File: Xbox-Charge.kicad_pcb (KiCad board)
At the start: 4 copper layers, 38.5 x 38.5 mm, 66 parts, among them J1 Conn_01x04_Pin, Q1 CSD17551Q3A, Q2 CSD17551Q3A, Q3 CSD17551Q3A, Q4 CSD17551Q3A, Q5 CSD25402Q3A, U2 BQ25713RSNR

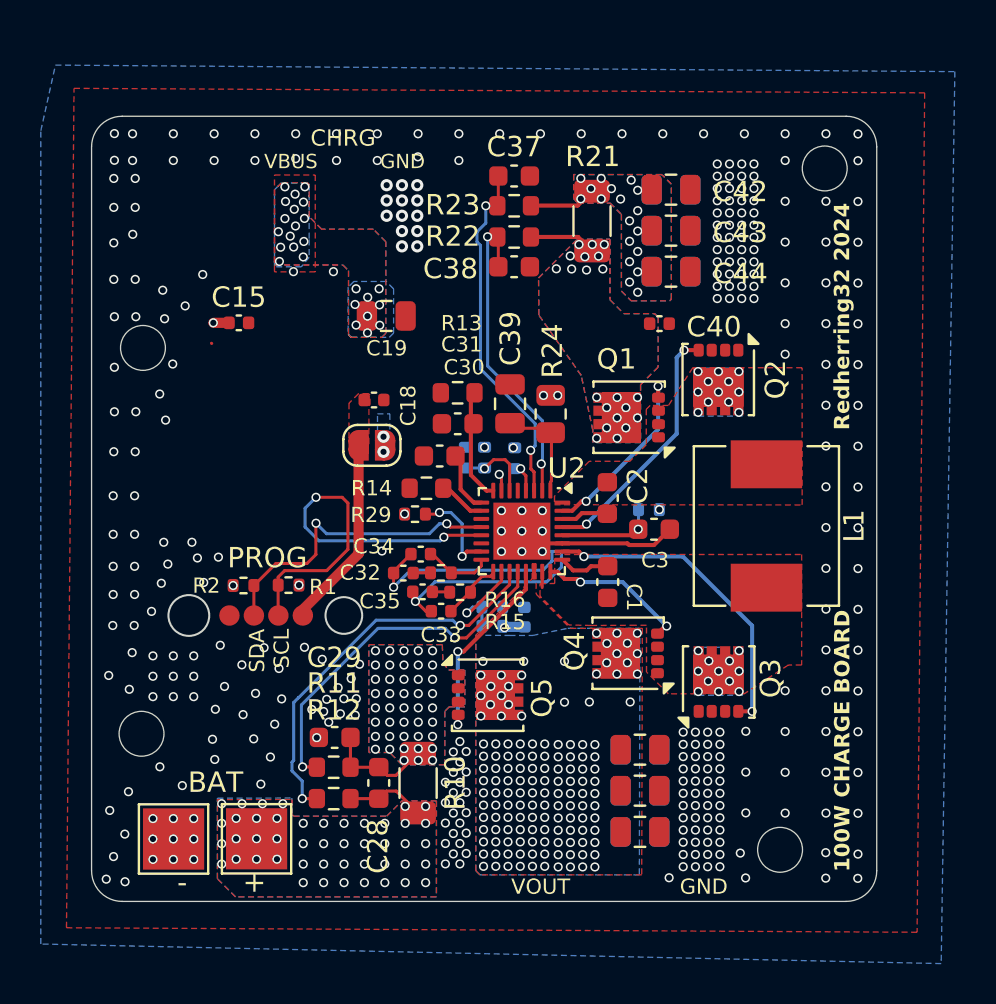
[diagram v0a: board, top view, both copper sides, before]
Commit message: Trim corner
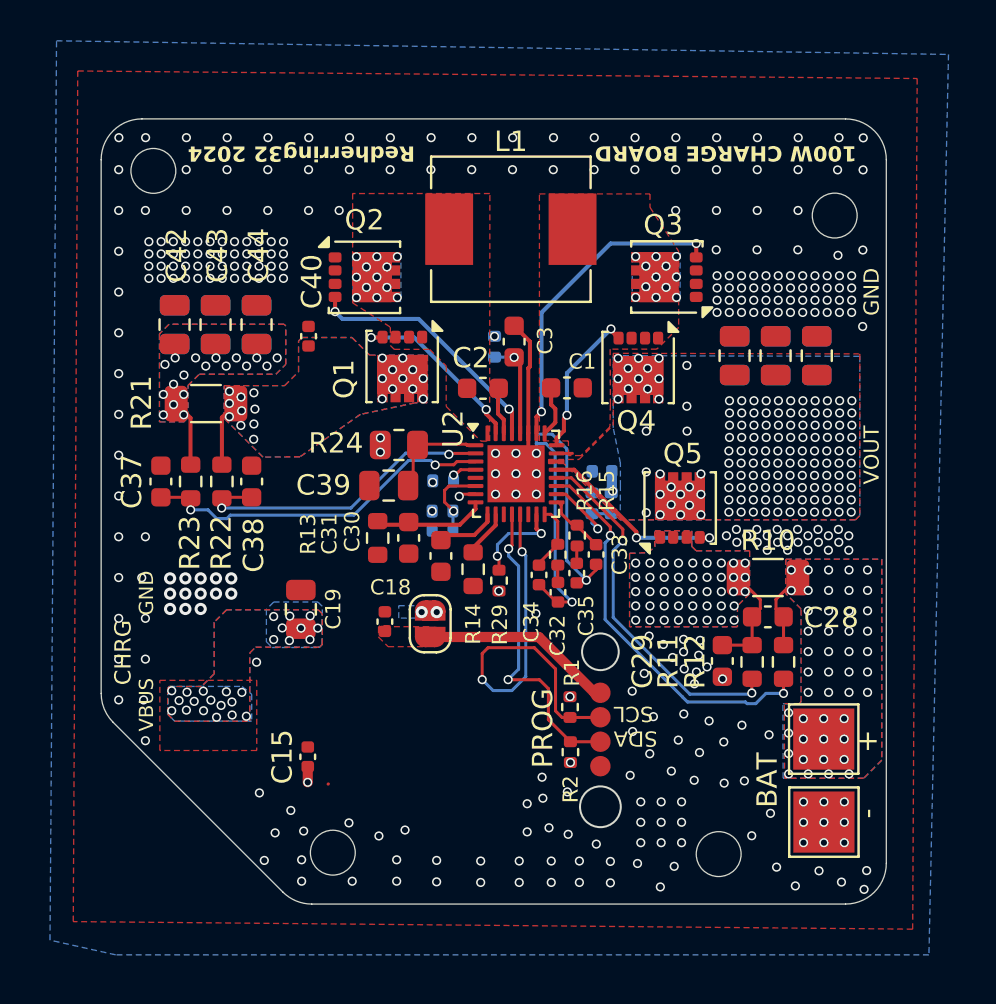
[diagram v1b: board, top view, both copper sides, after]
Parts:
- moved REF** 32.9 mm to (150.8, 33.3), turned to 90 degrees
- moved TP3 31.9 mm to (183.7, 65.2), turned to 90 degrees
- moved REF** 31.2 mm to (184.2, 35.5), turned to 90 degrees
- moved REF** 28.9 mm to (178.5, 66.8), turned to 90 degrees
- moved TP2 28.2 mm to (183.7, 61.2), turned to 90 degrees
- moved REF** 26.4 mm to (159.6, 66.7), turned to 90 degrees
- moved C42 25.2 mm to (151.8, 40.8), turned to 90 degrees
- moved C47 25.2 mm to (151.8, 40.8), turned to 90 degrees
- moved C12 24.9 mm to (183.3, 42.4), turned to 90 degrees
- moved C27 24.9 mm to (183.3, 42.4), turned to 90 degrees
- moved R12 23.1 mm to (181.7, 57.4), turned to -90 degrees
- moved C37 22.9 mm to (151.2, 48.5), turned to 90 degrees
- moved C43 22.8 mm to (153.9, 40.8), turned to 90 degrees
- moved C46 22.8 mm to (153.9, 40.8), turned to 90 degrees
- moved C13 22.4 mm to (181.3, 42.4), turned to 90 degrees
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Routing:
- net GND: vias 328 -> 311
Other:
- outline, holes or cut-outs redrawn
